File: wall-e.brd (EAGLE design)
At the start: 61.3 x 46.5 mm, 71 parts, among them IC1 VREG-TS1117CW-3V3, T1 BC847, U1 TSM2306CX, U2 TSM2306CX, U3 TSM2306CX, U4 TSM2306CX, U5 TSM2306CX, U6 TSM2306CX, U7 TSM2306CX, U8 LM293AD, U9 TSM2306CX

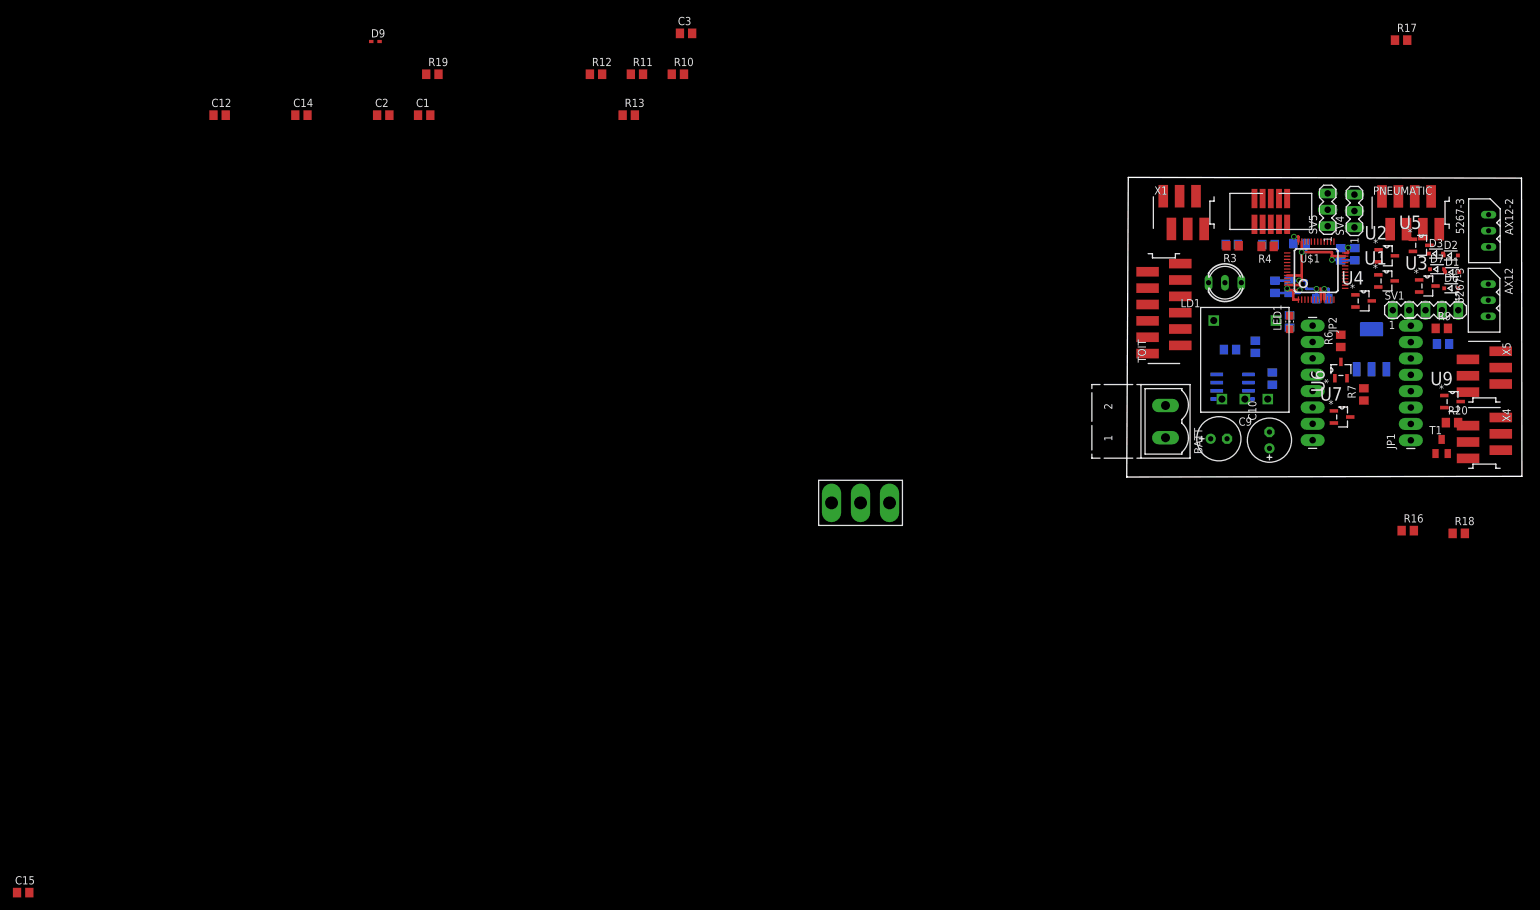
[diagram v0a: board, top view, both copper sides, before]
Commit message: Placement
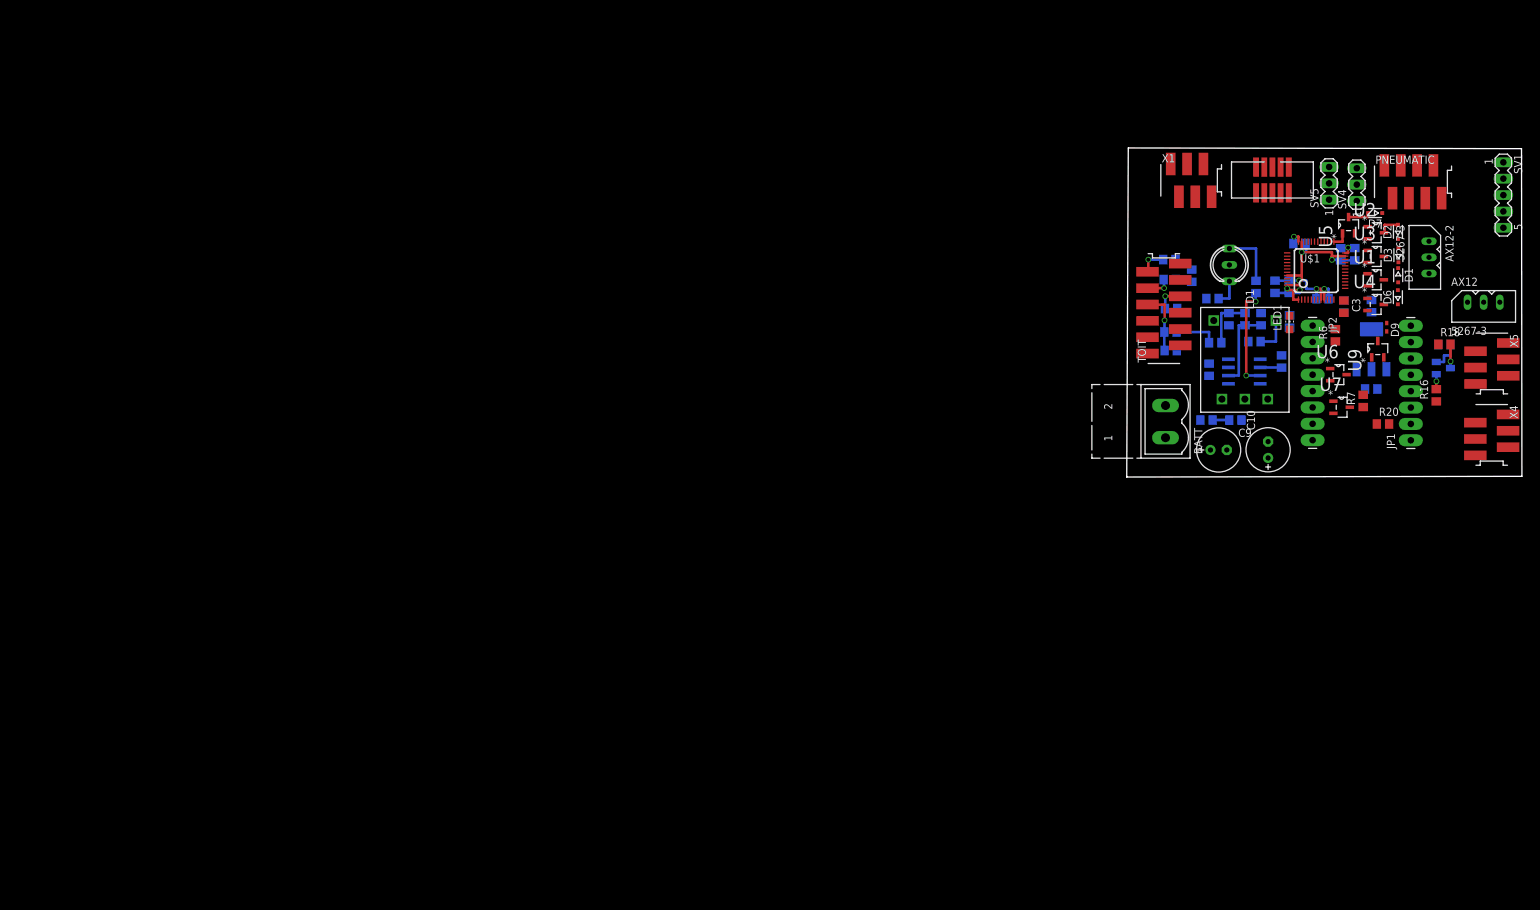
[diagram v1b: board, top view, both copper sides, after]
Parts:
- removed ON/OFF: SWITCH, switch:SWITCH
- added C16: 100nF, rcl:C0805
- moved C15 198.2 mm to (59.9, 40.0), flipped to the bottom, turned to 180 degrees
- moved C14 164.5 mm to (86.8, 44.0), flipped to the bottom, turned to 270 degrees
- moved D9 163.1 mm to (93.5, 40.8), turned to 270 degrees
- moved C12 158.5 mm to (66.9, 38.4), flipped to the bottom
- moved C2 156.2 mm to (91.1, 44.0), flipped to the bottom, turned to 90 degrees
- moved C1 153.0 mm to (91.1, 31.2), flipped to the bottom, turned to 180 degrees
- moved R19 122.3 mm to (60.0, 37.1), flipped to the bottom, turned to 180 degrees
- moved C3 110.6 mm to (86.8, 43.9), turned to 270 degrees
- moved R12 107.6 mm to (71.5, 42.0), flipped to the bottom, turned to 270 degrees
- moved R11 104.1 mm to (74.0, 42.0), flipped to the bottom, turned to 90 degrees
- moved R13 98.4 mm to (69.0, 42.0), flipped to the bottom, turned to 90 degrees
- moved R10 98.0 mm to (65.5, 26.4), flipped to the bottom
- moved R17 47.7 mm to (102.4, 38.1), flipped to the bottom, turned to 180 degrees
- moved R9 35.1 mm to (70.0, 26.3), flipped to the bottom
- moved R18 29.4 mm to (102.5, 38.1)
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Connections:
- removed net N$30: BATT.1, ON/OFF.P$3
- net +12V: now also BATT.1; no longer ON/OFF.P$1, ON/OFF.P$2
- net +3V3: no longer U8.8
- net +5V: now also C16.2, U8.8
- net GND: now also C16.1
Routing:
- net N$16: track 0.00 -> 16.5 mm, vias 0 -> 2
- net N$20: track 0.00 -> 12.9 mm
- net MCU_RESET: track 0.00 -> 9.88 mm, vias 0 -> 1
- net N$17: track 0.00 -> 9.15 mm
- net N$21: track 0.00 -> 8.27 mm
- net GND: track 37.4 -> 44.1 mm
- net N$19: track 0.00 -> 5.94 mm
- net N$13: track 0.00 -> 5.65 mm
- net N$25: track 0.00 -> 4.91 mm
- net N$15: track 0.00 -> 4.36 mm
- net N$1: track 0.00 -> 4.33 mm, vias 0 -> 1
- net N$4: track 0.00 -> 4.32 mm, vias 0 -> 1
- net N$3: track 0.00 -> 3.97 mm, vias 0 -> 1
- net AX12-TX: track 0.00 -> 3.70 mm, vias 0 -> 1
- net N$9: track 0.00 -> 3.64 mm
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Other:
- board size 61.3 x 46.5 mm -> 61.3 x 51.1 mm
